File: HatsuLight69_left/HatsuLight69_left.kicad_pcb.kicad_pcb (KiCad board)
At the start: 2 copper layers, 166.3 x 125.7 mm, 133 parts, among them J1 USB_C_Receptacle, J2 MJ-4PP-9, J3 I2C, J4 SPI, SW1 SW_PUSH, SW10 SW_PUSH-kbd, SW11 SW_PUSH-kbd, SW12 SW_PUSH-kbd, SW13 SW_PUSH-kbd, SW14 SW_PUSH-kbd, SW15 SW_PUSH-kbd, SW16 SW_PUSH-kbd, SW17 SW_PUSH-kbd, SW18 SW_PUSH-kbd, SW19 SW_PUSH-kbd, SW2 SW_PUSH-kbd, SW20 SW_PUSH-kbd, SW21 SW_PUSH-kbd, SW22 SW_PUSH-kbd, SW23 SW_PUSH-kbd, SW24 SW_PUSH-kbd, SW25 SW_PUSH-kbd, SW26 SW_PUSH-kbd, SW27 SW_PUSH-kbd, SW28 SW_PUSH-kbd, SW29 SW_PUSH-kbd, SW3 SW_PUSH-kbd, SW30 SW_PUSH-kbd, SW31 SW_PUSH-kbd, SW32 SW_PUSH-kbd, SW33 SW_PUSH-kbd, SW4 SW_PUSH-kbd, SW5 SW_PUSH-kbd, SW6 SW_PUSH-kbd, SW7 SW_PUSH-kbd, SW8 SW_PUSH-kbd, SW9 SW_PUSH-kbd, U1 ATMEGA32U4, X1 CSTNE16M0V530000R0

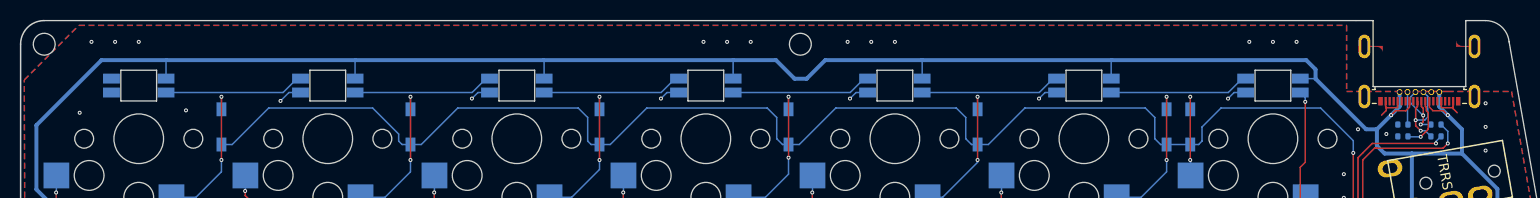
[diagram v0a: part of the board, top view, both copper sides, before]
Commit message: update
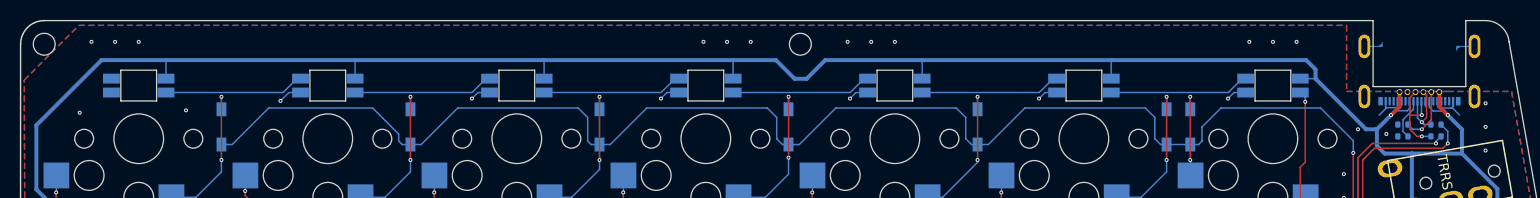
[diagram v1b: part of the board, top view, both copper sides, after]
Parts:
- J1: moved to B.Cu
- turned J1 to 0 degrees
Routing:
- net Net-(J1-PadB5): track 3.30 -> 5.81 mm, vias 0 -> 1
- net Net-(J1-PadA5): track 5.33 -> 4.26 mm, vias 1 -> 0
- net unconnected-(J1-PadA8): track 0.00 -> 0.50 mm
- net Net-(J1-PadA6): track 6.66 -> 6.69 mm, vias 2 -> 1
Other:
- outline, holes or cut-outs redrawn
